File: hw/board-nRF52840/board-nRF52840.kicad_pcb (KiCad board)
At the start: 2 copper layers, 30 x 42 mm, 17 parts, among them J1 JST-PH 2.0 / BATTERY, SW1 B3U-1000P, U1 XIAO nRF52840, U2 BMA400

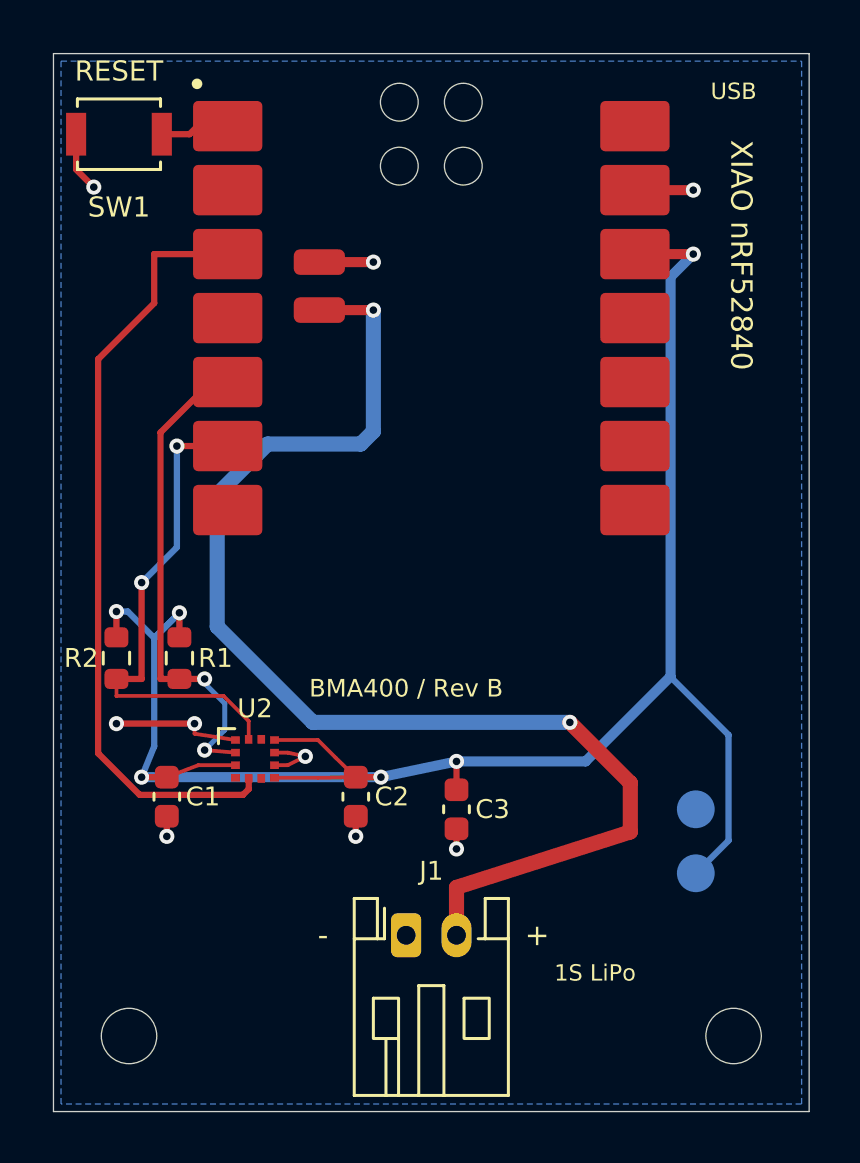
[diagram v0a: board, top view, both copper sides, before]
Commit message: Update PCB
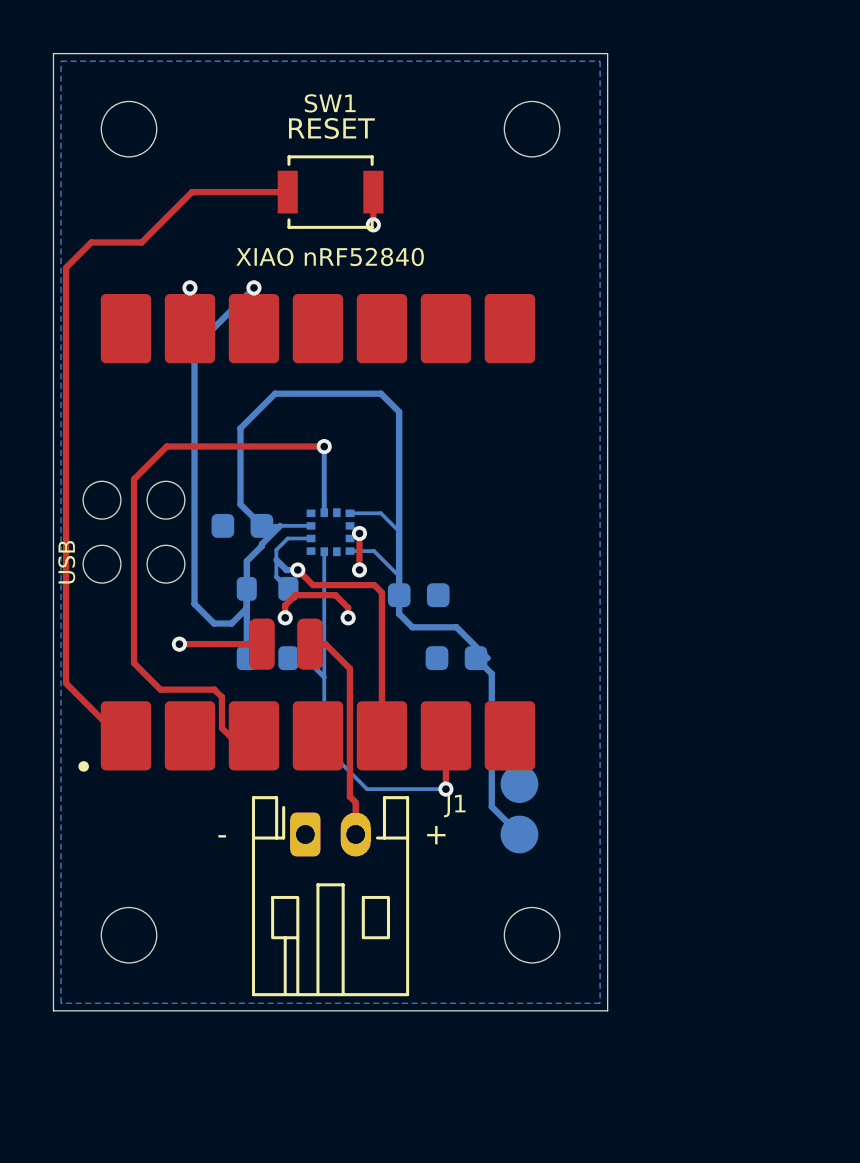
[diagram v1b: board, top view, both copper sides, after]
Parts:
- added H7: MountingHole_2.2mm_M2, Board:MountingHole_2.2mm_M2, F.Cu at (52.0, 53.0)
- added H8: MountingHole_2.2mm_M2, Board:MountingHole_2.2mm_M2, F.Cu at (68.0, 53.0)
- C1, C2, C3, R1, R2, U2: moved to B.Cu
- moved H3 21.8 mm to (50.9, 70.3), turned to 90 degrees
- moved H4 21.3 mm to (50.9, 67.7), turned to 90 degrees
- moved H5 18.3 mm to (53.5, 70.3), turned to 90 degrees
- moved H6 17.8 mm to (53.5, 67.7), turned to 90 degrees
- moved C1 11.2 mm to (56.5, 68.8), turned to 180 degrees
- moved U1 9.62 mm to (59.5, 69.0), turned to 90 degrees
- moved U2 9.49 mm to (60.0, 69.0)
- moved H2 8.94 mm to (68.0, 85.0)
- moved SW1 8.71 mm to (60.0, 55.5), turned to 0 degrees
- moved C2 8.38 mm to (63.5, 71.5), turned to 0 degrees
- moved TP1 7.17 mm to (67.5, 81.0)
- moved TP2 7.07 mm to (67.5, 79.0)
- moved C3 6.00 mm to (65.0, 74.0), turned to 180 degrees
- moved R2 6.00 mm to (57.5, 74.0), turned to 0 degrees
- moved J1 5.66 mm to (59.0, 81.0)
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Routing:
- net /VBAT: track 49.5 -> 8.67 mm, vias 2 -> 0
- net /FACTORY_RESET: track 2.75 -> 29.8 mm
- net /+3V3: track 76.6 -> 62.7 mm, vias 6 -> 1
- net /ACC_INT1: track 30.8 -> 24.7 mm, vias 0 -> 1
- net /I2C_SDA: track 19.7 -> 13.7 mm, vias 2 -> 1
- net /GND: track 16.9 -> 11.4 mm, vias 9 -> 7
- net /I2C_SCL: track 19.9 -> 17.1 mm, vias 2 -> 1
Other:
- board size 30 x 42 mm -> 22 x 38 mm
- board text added: "22 x 38 mm / 2 layers / 1.6 mm FR4"
- board text added: "BMA400 / Rev C"
- board text added: "nRF52840 / Rev C"
- board text removed: "1S LiPo"
- board text removed: "30 x 42 mm / 2 layers / 1.6 mm FR4"
- board text removed: "BMA400 / Rev B"
- board text removed: "board-nRF52840 / SMD"
